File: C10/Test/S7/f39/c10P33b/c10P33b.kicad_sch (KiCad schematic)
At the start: 5 parts

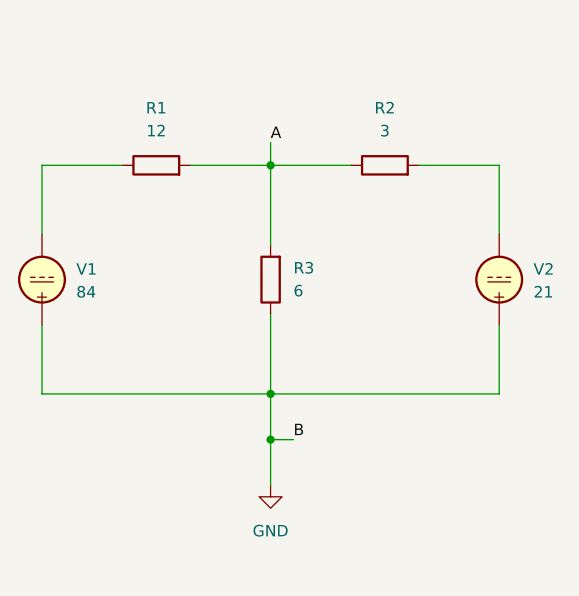
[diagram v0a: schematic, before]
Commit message: additiona upload Chapter 10
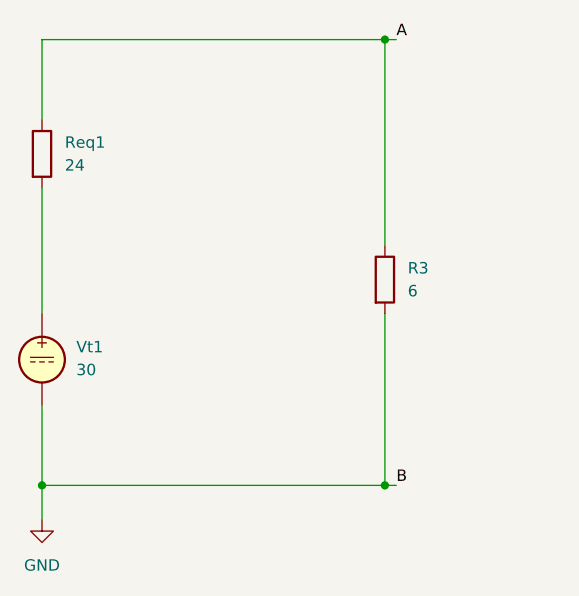
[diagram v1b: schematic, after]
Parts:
- removed R1: 12, symbol Device:R
- removed R2: 3, symbol Device:R
- removed V1: 84, symbol Simulation_SPICE:VDC
- removed V2: 21, symbol Simulation_SPICE:VDC
- added Req1: 24, symbol Device:R
- added Vt1: 30, symbol Simulation_SPICE:VDC
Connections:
- net A: now also R3.1, Req1.1; no longer R3.2
- net GND: now also R3.2, Vt1.2; no longer R3.1
- new net: Req1.2, Vt1.1
